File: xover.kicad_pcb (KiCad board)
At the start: 2 copper layers, 100 x 100 mm, 196 parts, among them J1 Screw_Terminal_01x04, J10 Conn_02x03_Odd_Even, J11 Conn_02x03_Odd_Even, J12 Conn_02x03_Odd_Even, J13 Conn_02x03_Odd_Even, J14 Conn_02x03_Odd_Even, J2 Conn_02x03_Odd_Even, J3 Screw_Terminal_01x02, J4 Conn_02x03_Odd_Even, J5 Screw_Terminal_01x04, J6 Screw_Terminal_01x04, J7 Screw_Terminal_01x03, J8 Conn_02x03_Odd_Even, J9 Conn_01x04_Male, U1 NE5532, U10 NE5532, U11 NE5532, U12 NE5532, U13 NE5532, U2 NE5532, U3 NE5532, U4 NE5532, U5 NE5532, U6 NE5532, U7 NE5532, U8 NE5532, U9 NE5532

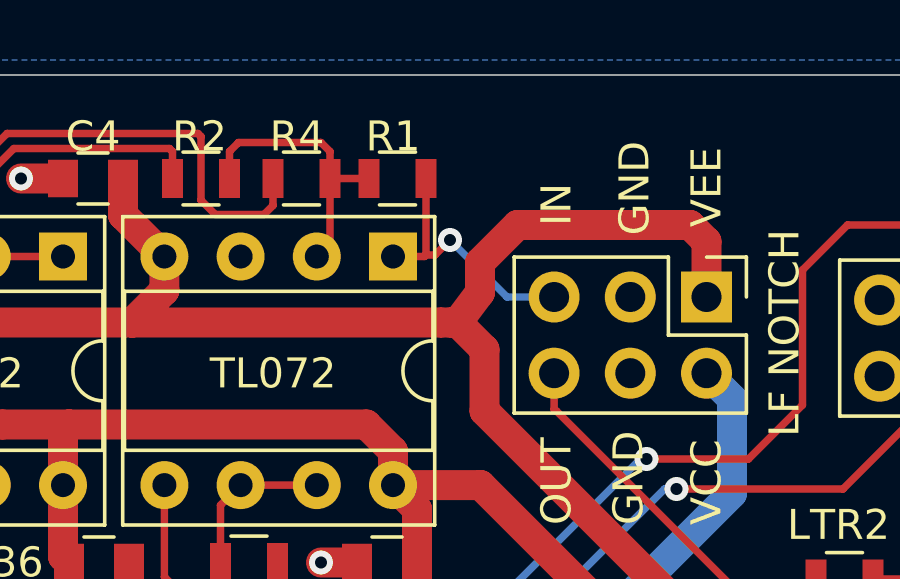
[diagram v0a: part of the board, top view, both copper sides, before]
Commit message: created gerbers
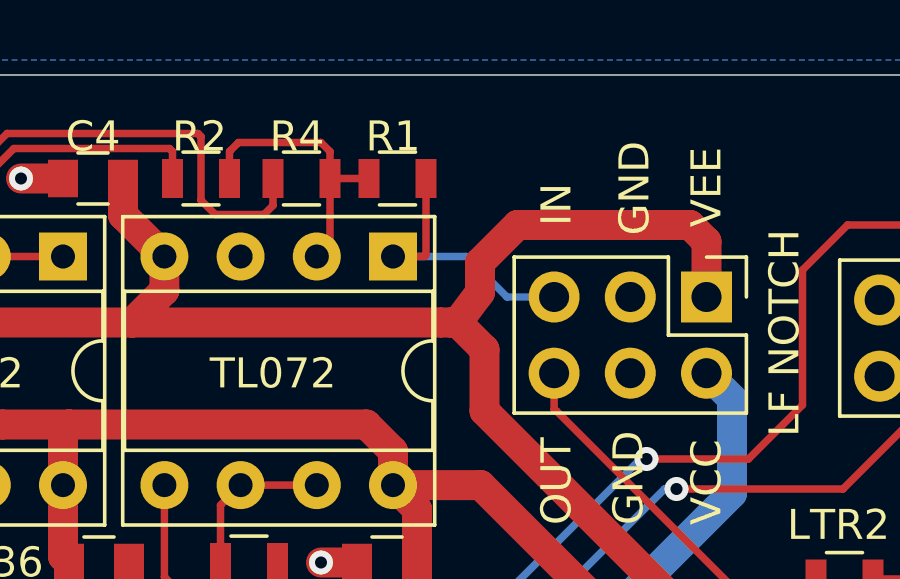
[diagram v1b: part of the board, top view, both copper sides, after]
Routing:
- net /notch/IN: track 8.93 -> 9.60 mm, vias 1 -> 0
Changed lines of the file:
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@@
     (thickness 1.6)
     (drawings 89)
-    (tracks 1305)
+    (tracks 1303)
     (zones 0)
     (modules 196)
@@
       (outputformat 1)
       (mirror false)
-      (drillshape 1)
+      (drillshape 0)
       (scaleselection 1)
-      (outputdirectory ""))
+      (outputdirectory "plot"))
   )
   (net 0 "")
@@
   (segment (start 121 104.8) (end 117.8 104.8) (width 0.25) (layer F.Cu) (net 30))
   (segment (start 112.8 104.2) (end 113 104.2) (width 0.25) (layer F.Cu) (net 30))
-  (segment (start 110.6 106.1) (end 110.9 106.1) (width 0.25) (layer F.Cu) (net 68))
   (segment (start 113.6 104.8) (end 113 104.2) (width 0.25) (layer F.Cu) (net 30))
   (segment (start 117.8 104.8) (end 113.6 104.8) (width 0.25) (layer F.Cu) (net 30))
@@
   (segment (start 114.4 108.6) (end 117.6 108.6) (width 0.25) (layer F.Cu) (net 31))
   (segment (start 117.8 108.8) (end 121 108.8) (width 0.25) (layer F.Cu) (net 31))
-  (segment (start 106.8 121.1) (end 106.8 119.4) (width 0.25) (layer F.Cu) (net 32))
-  (segment (start 106.8 122.6) (end 106.8 121.1) (width 0.25) (layer F.Cu) (net 32))
   (segment (start 116.9 111.2) (end 116.9 111.5) (width 0.25) (layer F.Cu) (net 31))
   (segment (start 117.1 109.5) (end 117.8 108.8) (width 0.25) (layer F.Cu) (net 31))
   (segment (start 116.9 109.7) (end 117.8 108.8) (width 0.25) (layer F.Cu) (net 31))
   (segment (start 116.9 111.2) (end 116.9 109.7) (width 0.25) (layer F.Cu) (net 31))
+  (segment (start 106.8 121.1) (end 106.8 119.4) (width 0.25) (layer F.Cu) (net 32))
+  (segment (start 106.8 122.6) (end 106.8 121.1) (width 0.25) (layer F.Cu) (net 32))
   (segment (start 118.8 113.4) (end 118.8 111.2) (width 0.25) (layer F.Cu) (net 32))
   (segment (start 118.8 113.8) (end 118.8 113.4) (width 0.25) (layer F.Cu) (net 32))
@@
   (segment (start 85 64.8) (end 88.9 64.8) (width 0.25) (layer F.Cu) (net 67))
   (segment (start 81.1 68.7) (end 85 64.8) (width 0.25) (layer F.Cu) (net 67))
+  (segment (start 110.6 106.1) (end 110.9 106.1) (width 0.25) (layer F.Cu) (net 68))
   (segment (start 105.45137 80.42) (end 106.86 80.42) (width 0.25) (layer F.Cu) (net 68))
   (segment (start 104.32 80.42) (end 105.45137 80.42) (width 0.25) (layer F.Cu) (net 68))
@@
   (segment (start 84.45 31) (end 84.4 31.05) (width 0.25) (layer F.Cu) (net 73))
   (segment (start 84.45 28.45) (end 84.45 31) (width 0.25) (layer F.Cu) (net 73))
-  (via (at 85.25 30.5) (size 0.8) (drill 0.4) (layers F.Cu B.Cu) (net 73))
-  (segment (start 87.15 32.4) (end 85.25 30.5) (width 0.25) (layer B.Cu) (net 73))
   (segment (start 88.72 32.4) (end 87.15 32.4) (width 0.25) (layer B.Cu) (net 73))
-  (segment (start 84.75 31) (end 84.45 31) (width 0.25) (layer F.Cu) (net 73))
-  (segment (start 85.25 30.5) (end 84.75 31) (width 0.25) (layer F.Cu) (net 73))
+  (segment (start 85.8 31.05) (end 87.15 32.4) (width 0.25) (layer B.Cu) (net 73))
+  (segment (start 83.35 31.05) (end 85.8 31.05) (width 0.25) (layer B.Cu) (net 73))
   (segment (start 81.15 30.71) (end 80.81 31.05) (width 0.25) (layer F.Cu) (net 74))
   (segment (start 77.9 27.55) (end 78.2 27.25) (width 0.25) (layer F.Cu) (net 74))
